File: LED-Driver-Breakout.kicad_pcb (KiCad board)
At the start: 6 copper layers, 98 x 100 mm, 27 parts, among them U1 V10P45-M3/86A, U2 TSR0.5-2418

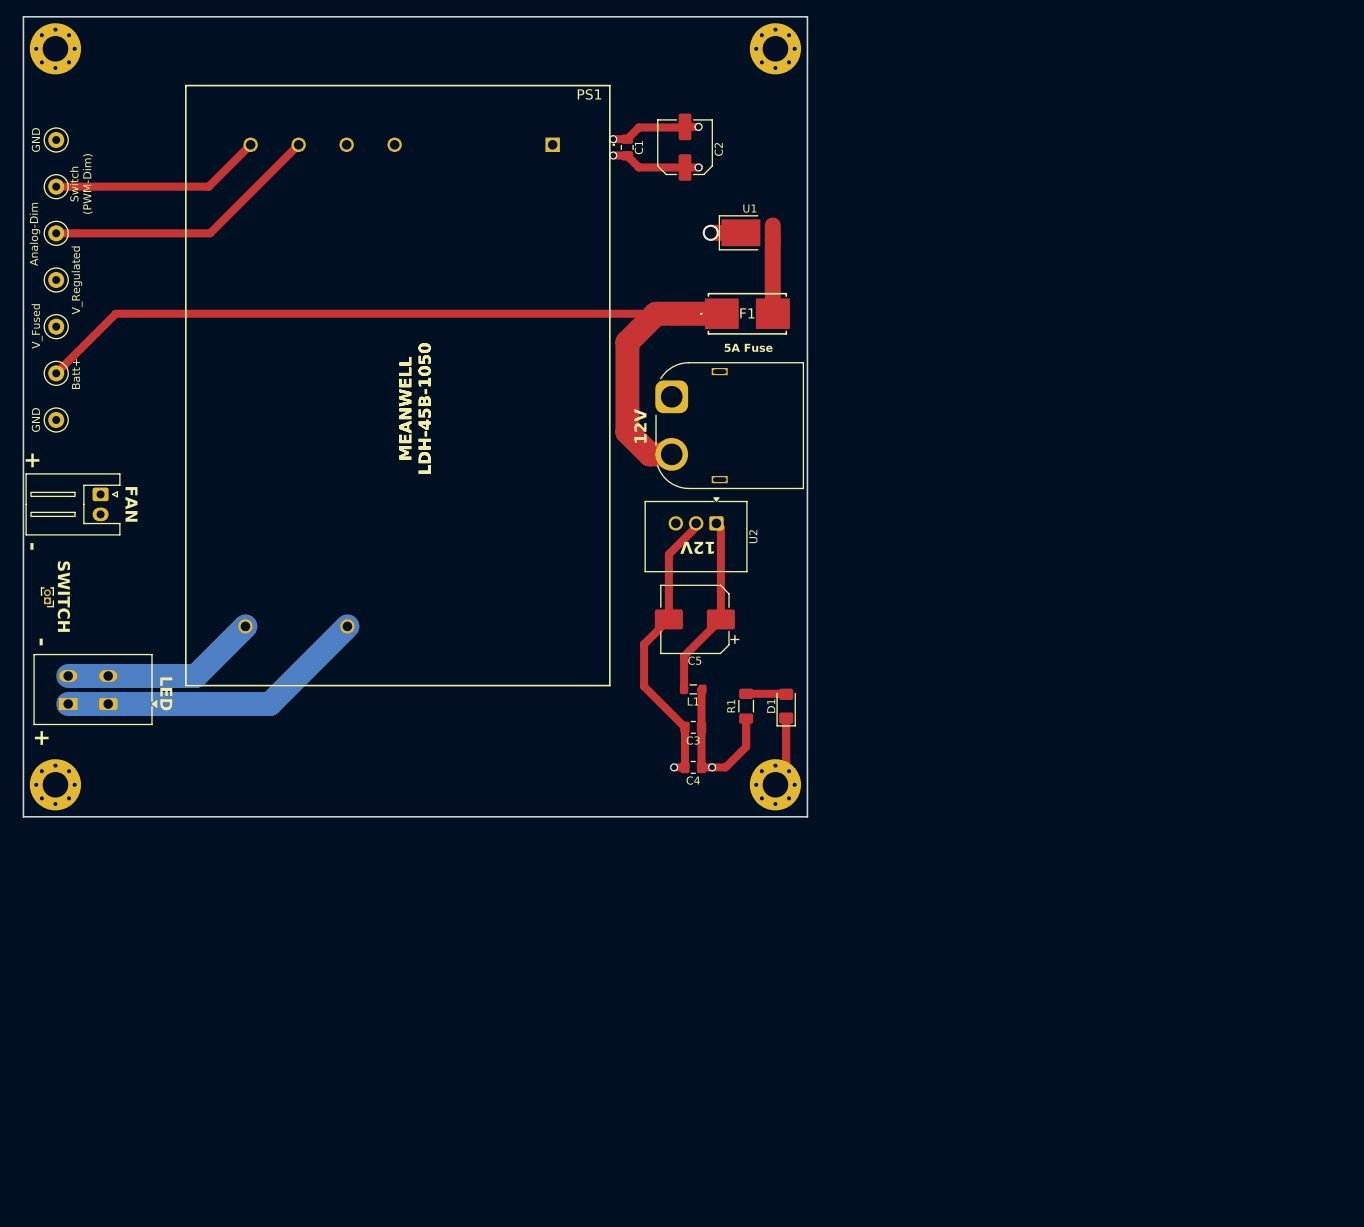
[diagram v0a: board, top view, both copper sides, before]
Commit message: forgot to add switch trace
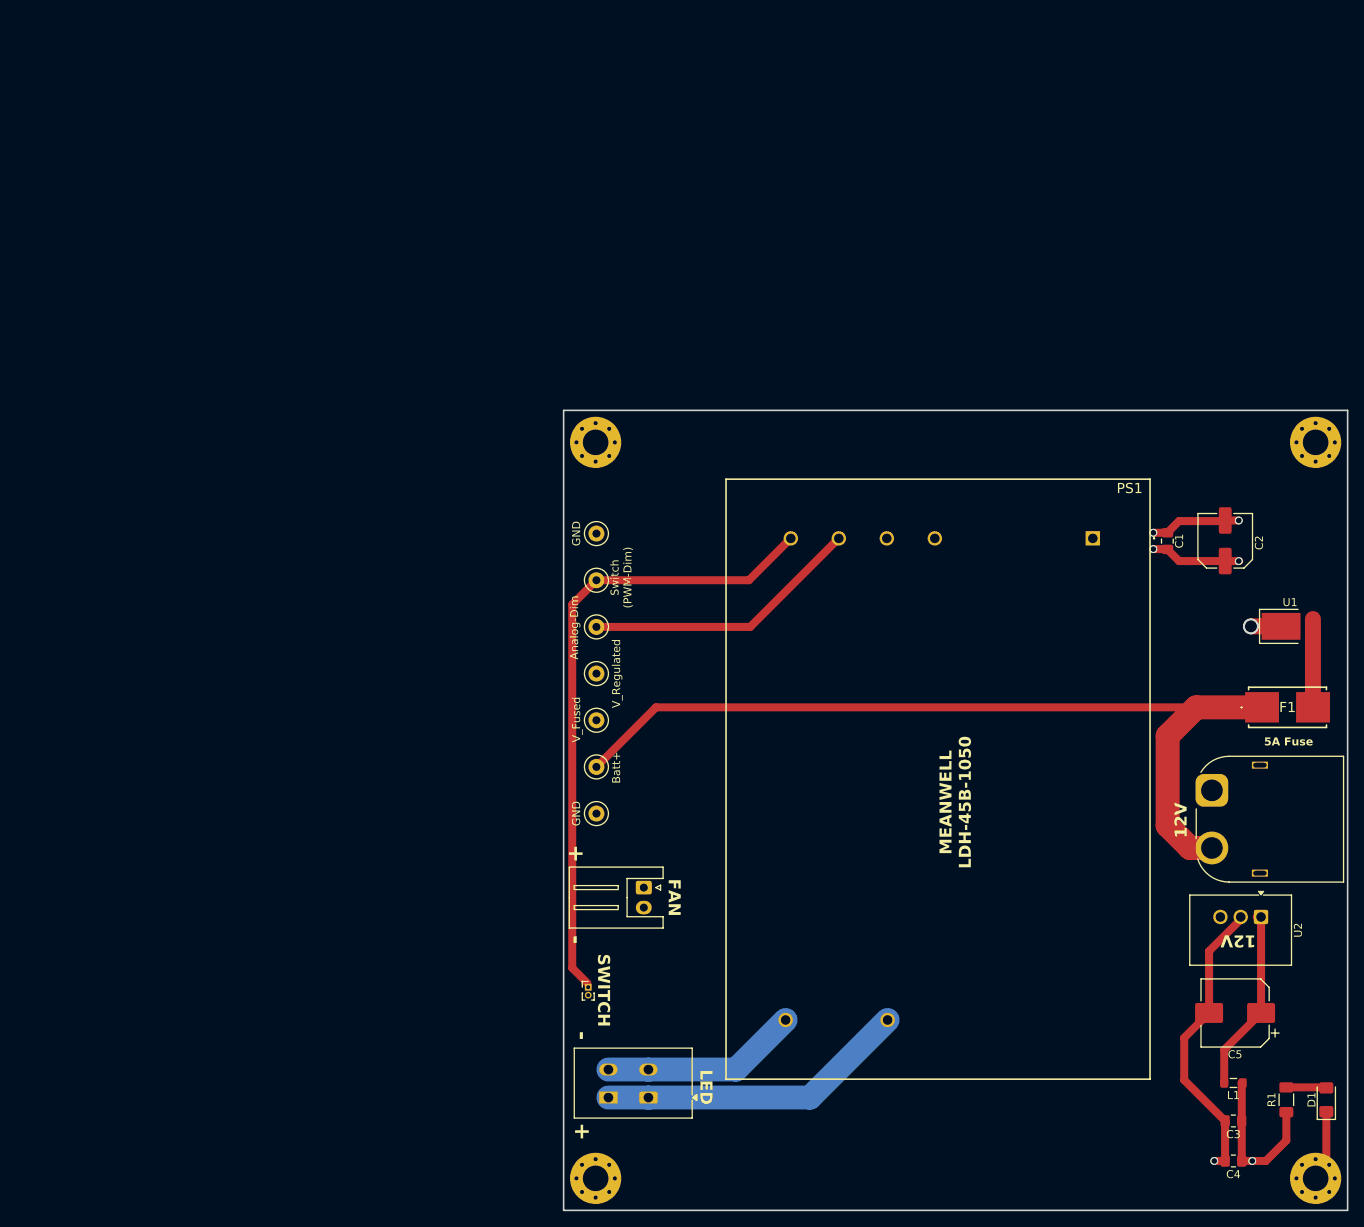
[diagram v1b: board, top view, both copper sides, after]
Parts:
- moved U2 84.0 mm to (154.7, 112.5)
- moved   83.8 mm to (77.5, 108.8)
- moved Analog-Dim 83.5 mm to (71.6, 76.3)
- moved D1 83.5 mm to (162.9, 135.4)
- moved R1 83.5 mm to (157.9, 135.4)
- moved Switch(PWM-Dim) 83.5 mm to (71.6, 70.4)
- moved V_Fused 83.5 mm to (71.6, 87.9)
- moved   83.5 mm to (161.5, 53.2)
- moved   83.5 mm to (161.5, 145.2)
- moved Batt+ 83.5 mm to (71.6, 93.8)
- moved C1 83.5 mm to (143.0, 65.5)
- moved C5 83.5 mm to (151.5, 124.5)
- moved GND 83.5 mm to (71.6, 99.6)
- moved GND 83.5 mm to (71.6, 64.6)
- moved REF** 83.5 mm to (78.1, 135.1)
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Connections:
- REF** pad 1: (no net) -> /switch
- REF** pad 2: (no net) -> GND
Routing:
- net /switch: track 26.8 -> 79.2 mm
